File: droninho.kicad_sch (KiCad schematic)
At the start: 27 parts, among them J1 Conn_01x02_Pin, J2 M2, J3 M1, J4 M3, J5 M4, J6 I2C, J7 TXD0/RXD0, J8 I2C, Q1 SI2300, Q2 SI2300, Q3 SI2300, Q4 SI2300, U1 ESP32 Dev Kit, U2 AMS1117-3.3, U4 MPU9250/6500

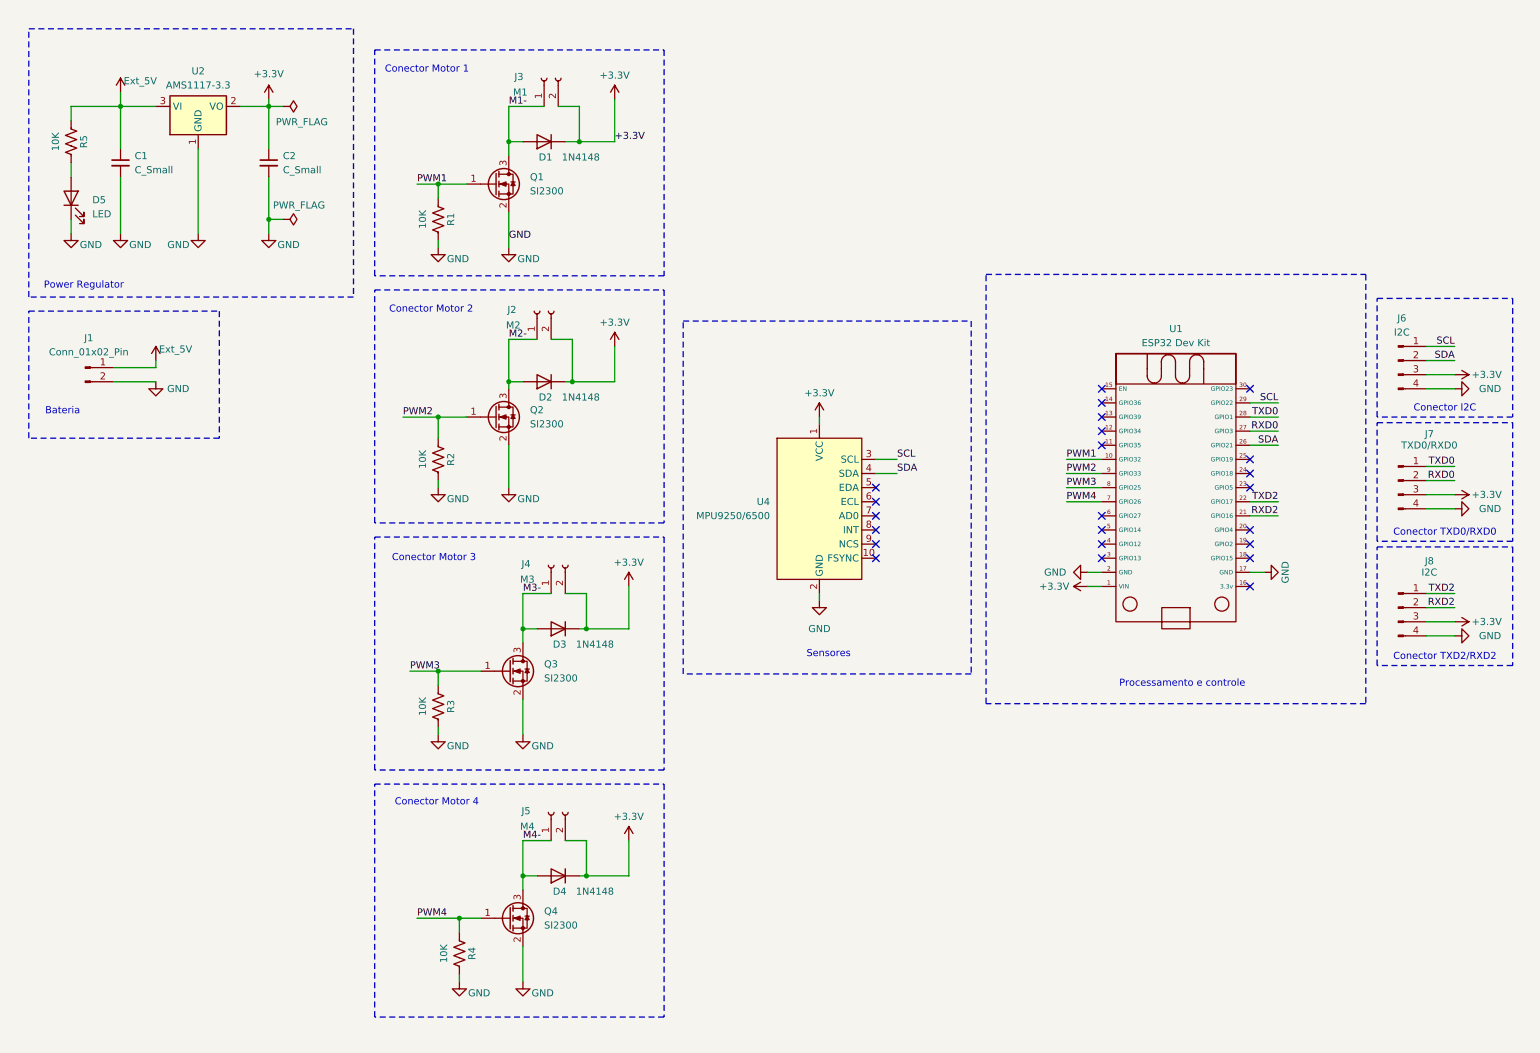
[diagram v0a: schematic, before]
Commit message: ERC done!
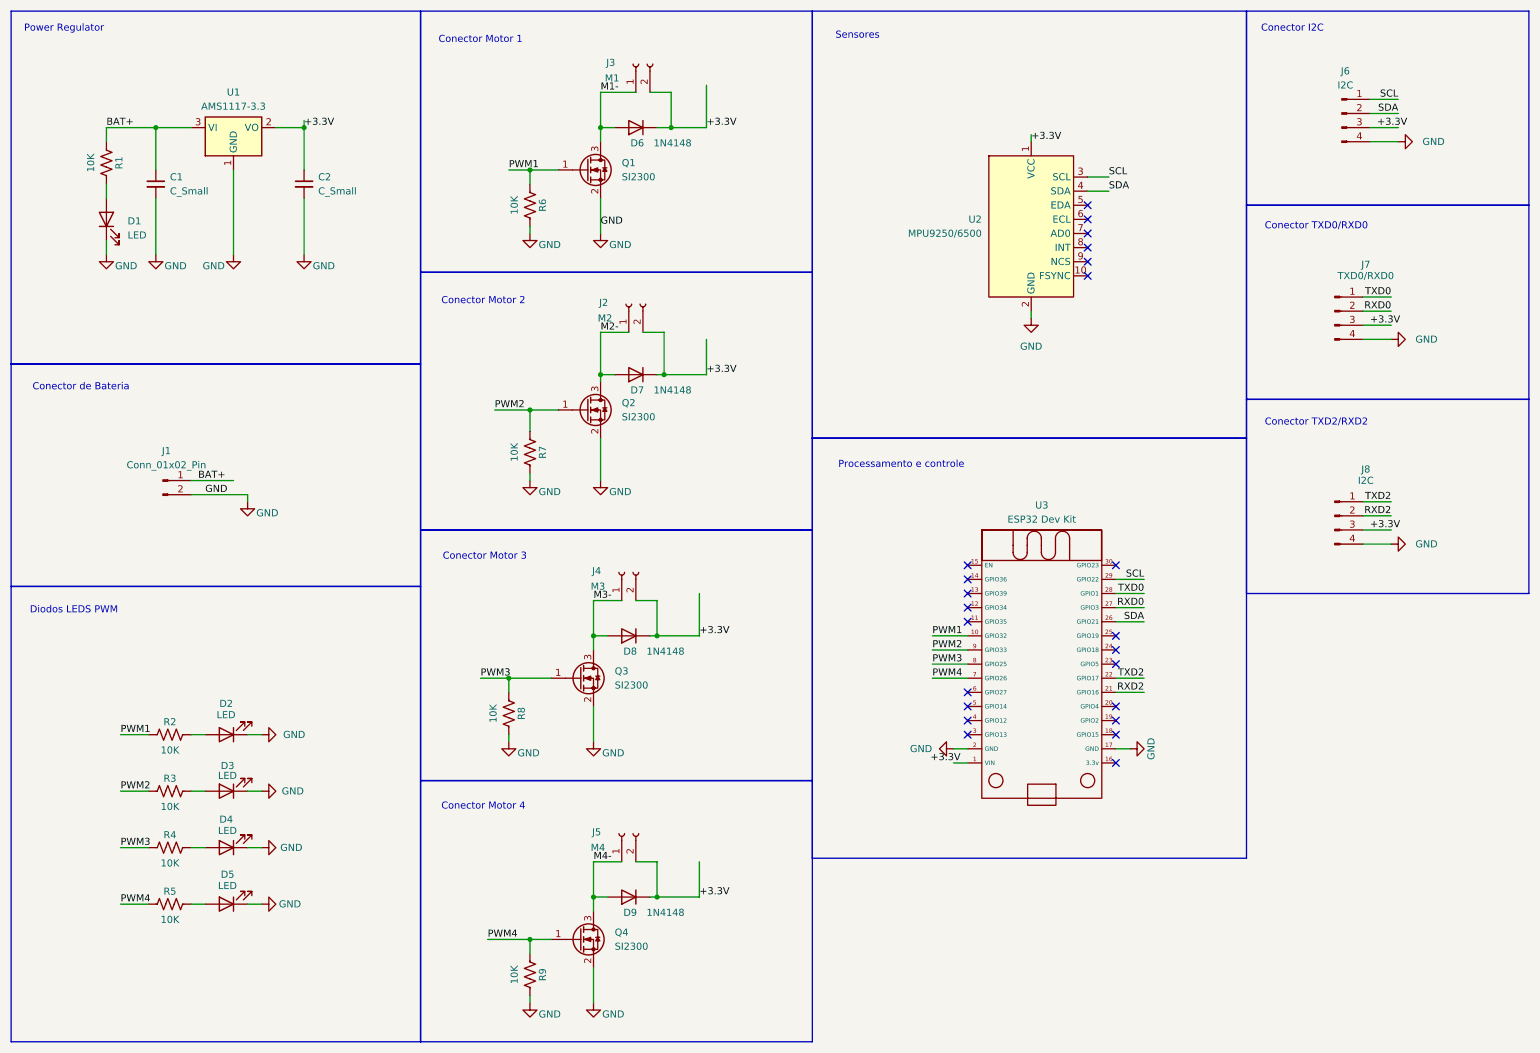
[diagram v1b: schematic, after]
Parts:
- added D2, D3, D4, D5: LED, LED_SMD:LED_0805_2012Metric_Pad1.15x1.40mm_HandSolder, symbol Device:LED
- added R2, R3, R4, R5: 10K, Resistor_SMD:R_0805_2012Metric_Pad1.20x1.40mm_HandSolder, symbol Device:R_US
- renumbered D5 to D1, D1 to D6, D2 to D7, D3 to D8, D4 to D9, R5 to R1, R1 to R6, R2 to R7, R3 to R8, R4 to R9, U2 to U1, U4 to U2, U1 to U3
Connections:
- net GND: now also D2.1 (K), D3.1 (K), D4.1 (K), D5.1 (K)
- net PWM1: now also R2.1
- net PWM2: now also R3.1
- net PWM3: now also R4.1
- net PWM4: now also R5.1
- net Ext_5V renamed BAT+
- new net: D2.2 (A), R2.2
- new net: D3.2 (A), R3.2
- new net: D4.2 (A), R4.2
- new net: D5.2 (A), R5.2
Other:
- note added: "Conector de Bateria"
- note added: "Diodos LEDS PWM"
- note removed: "Bateria"
- moved on the sheet: C1, C2, D1, D6, D7, D8, D9, J1, J2, J3, J4, J5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
